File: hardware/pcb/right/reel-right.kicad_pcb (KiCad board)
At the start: 2 copper layers, 145 x 88.1 mm, 47 parts, among them J1 Conn_01x02, J3 Conn_01x05, SW1 SW_Push, SW10 SW_Push, SW11 SW_Push, SW12 SW_Push, SW13 SW_Push, SW14 SW_Push, SW15 SW_Push, SW16 SW_Push, SW17 SW_Push, SW18 SW_Push, SW19 SW_Push, SW2 SW_Push, SW22 SW_SPDT, SW3 SW_Push, SW4 SW_Push, SW5 SW_Push, SW6 SW_Push, SW7 SW_Push, SW8 SW_Push, SW9 SW_Push

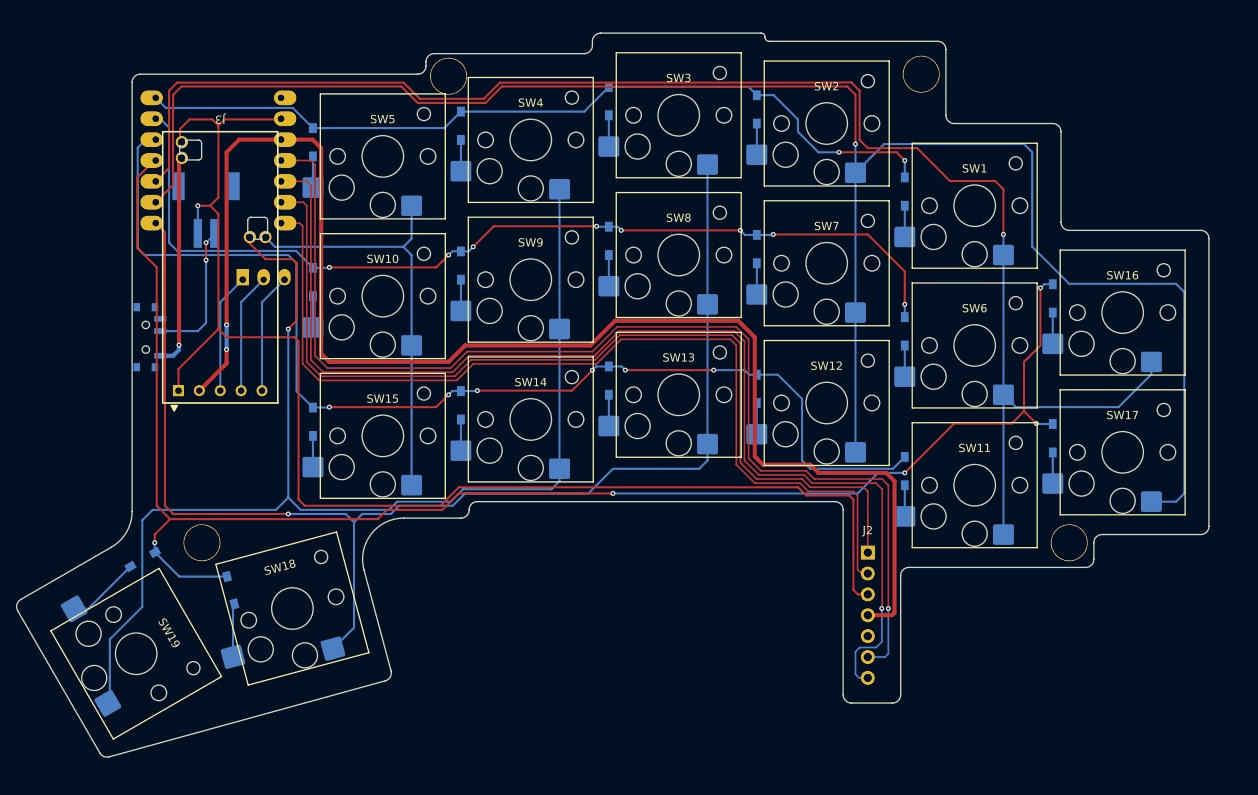
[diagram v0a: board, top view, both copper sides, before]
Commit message: Publish current hardware and fabrication assets
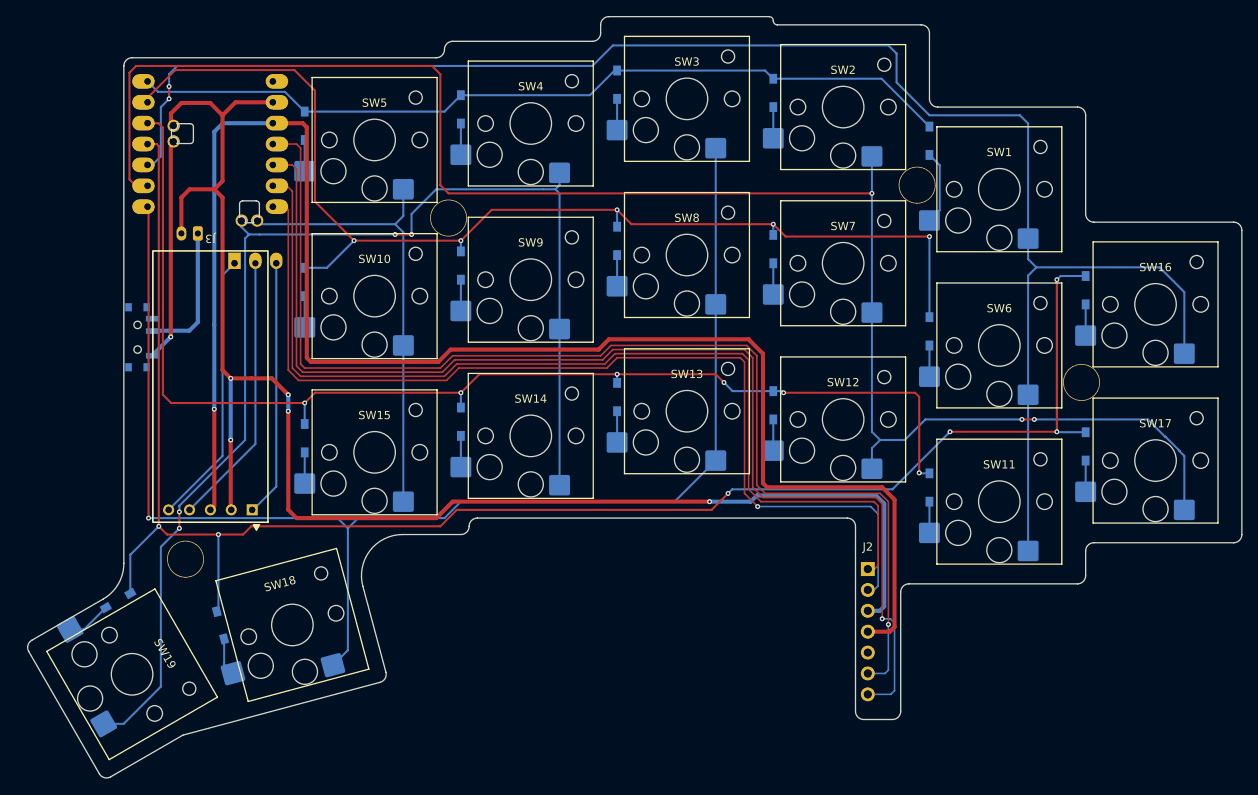
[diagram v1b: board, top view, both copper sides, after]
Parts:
- J1: footprint reel:JST_S2B-PH-SM4-TB -> Connector_JST:JST_PH_S2B-PH-K_1x02_P2.00mm_Horizontal
- moved Ref** 19.6 mm to (165.0, 88.0)
- moved Ref** 17.2 mm to (88.0, 68.0)
- moved J3 14.5 mm to (59.0, 103.5)
- moved Ref** 13.5 mm to (145.0, 64.0)
- moved D1 6.87 mm to (146.5, 55.8)
- moved D19 5.83 mm to (50.2, 113.1)
- moved D18 4.43 mm to (59.5, 114.8)
- moved D16 4.12 mm to (165.5, 74.0)
- moved D17 4.12 mm to (165.5, 93.0)
- moved SW16 4.12 mm to (174.0, 78.5)
- moved SW17 4.12 mm to (174.0, 97.5)
- moved D11 3.61 mm to (146.5, 98.0)
- moved SW1 3.61 mm to (155.0, 64.5)
- moved SW11 3.61 mm to (155.0, 102.5)
- moved D6 3.00 mm to (146.5, 79.0)
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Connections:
- J3 pad 1: GND -> SI
- J3 pad 2: 3.3V -> SCK
- J3 pad 3: SI -> 3.3V
- J3 pad 4: SCK -> GND
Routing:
- net Col1: track 227.5 -> 205.8 mm, vias 1 -> 3
- net Row1: track 116.8 -> 138.3 mm, vias 8 -> 5
- net 3.3V: track 176.1 -> 195.3 mm, vias 2 -> 1
- net GND: track 166.7 -> 185.5 mm, vias 1 -> 5
- net SI: track 14.6 -> 33.3 mm
- net SCK: track 14.6 -> 33.3 mm
- net CS: track 14.6 -> 31.3 mm
- net Col0: track 187.9 -> 204.0 mm, vias 1 -> 2
- net Row3: track 192.2 -> 207.3 mm, vias 5 -> 6
- net Col2: track 157.2 -> 167.7 mm
- net Row2: track 137.5 -> 145.5 mm
- net nCS: track 116.8 -> 122.4 mm, vias 0 -> 1
- net SCLK: track 117.2 -> 122.5 mm
- net Net-(D1-A): track 3.80 -> 9.01 mm
- net MOTION: track 140.4 -> 144.1 mm
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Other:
- board size 145 x 88.1 mm -> 147.7 x 92.6 mm
